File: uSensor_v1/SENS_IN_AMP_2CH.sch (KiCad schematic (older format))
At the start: 19 parts, among them U16 TBD

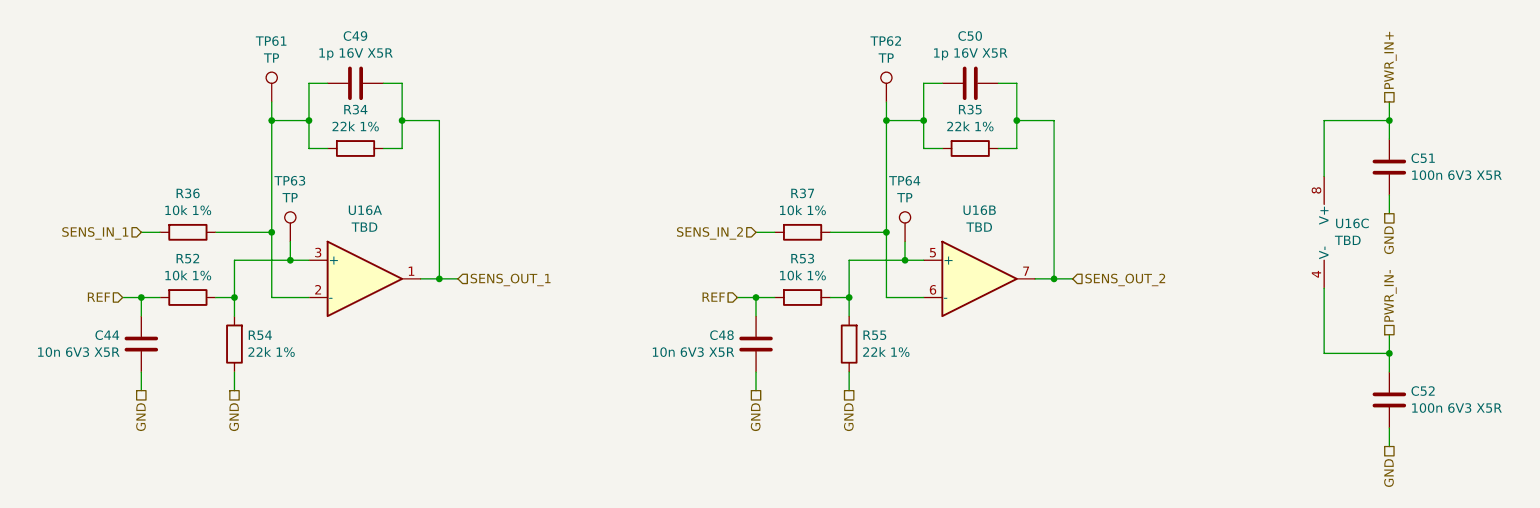
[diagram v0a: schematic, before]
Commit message: Layout in progress.
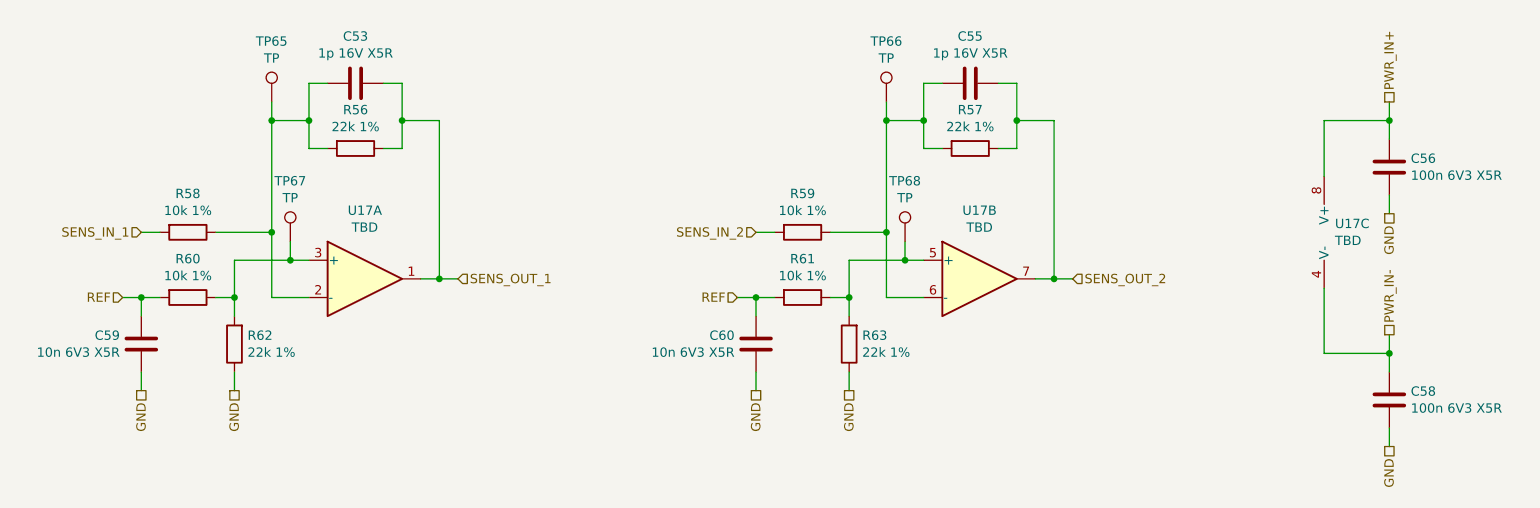
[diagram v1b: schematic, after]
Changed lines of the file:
@@
 AR Path="/5CFE311F/5C6F0205" Ref="R52"  Part="1"
 AR Path="/5E594B34/5C6F0205" Ref="R60"  Part="1"
-F 0 "R52" V 2443 3950 50  0000 C CNN
+F 0 "R60" V 2443 3950 50  0000 C CNN
 F 1 "10k 1%" V 2534 3950 50  0000 C CNN
 F 2 "Resistor_SMD:R_0603_1608Metric_Pad1.05x0.95mm_HandSolder" V 2580 3950 50  0001 C CNN
@@
 AR Path="/5CFE311F/5C6F020C" Ref="C49"  Part="1"
 AR Path="/5E594B34/5C6F020C" Ref="C53"  Part="1"
-F 0 "C49" V 3298 2800 50  0000 C CNN
+F 0 "C53" V 3298 2800 50  0000 C CNN
 F 1 "1p 16V X5R" V 3389 2800 50  0000 C CNN
 F 2 "Capacitor_SMD:C_0603_1608Metric_Pad1.05x0.95mm_HandSolder" H 3588 2650 50  0001 C CNN
@@
 AR Path="/5CFE311F/5C6F0213" Ref="R54"  Part="1"
 AR Path="/5E594B34/5C6F0213" Ref="R62"  Part="1"
-F 0 "R54" H 2830 4154 50  0000 R CNN
+F 0 "R62" H 2830 4154 50  0000 R CNN
 F 1 "22k 1%" H 2830 4245 50  0000 R CNN
 F 2 "Resistor_SMD:R_0603_1608Metric_Pad1.05x0.95mm_HandSolder" V 2830 4200 50  0001 C CNN
@@
 AR Path="/5CFE311F/5C6F0221" Ref="R36"  Part="1"
 AR Path="/5E594B34/5C6F0221" Ref="R58"  Part="1"
-F 0 "R36" V 2443 3600 50  0000 C CNN
+F 0 "R58" V 2443 3600 50  0000 C CNN
 F 1 "10k 1%" V 2534 3600 50  0000 C CNN
 F 2 "Resistor_SMD:R_0603_1608Metric_Pad1.05x0.95mm_HandSolder" V 2580 3600 50  0001 C CNN
@@
 AR Path="/5CFE311F/5C6F0228" Ref="R34"  Part="1"
 AR Path="/5E594B34/5C6F0228" Ref="R56"  Part="1"
-F 0 "R34" V 3343 3150 50  0000 C CNN
+F 0 "R56" V 3343 3150 50  0000 C CNN
 F 1 "22k 1%" V 3434 3150 50  0000 C CNN
 F 2 "Resistor_SMD:R_0603_1608Metric_Pad1.05x0.95mm_HandSolder" V 3480 3150 50  0001 C CNN
@@
 AR Path="/5CFE311F/5D2C6388" Ref="TP61"  Part="1"
 AR Path="/5E594B34/5D2C6388" Ref="TP65"  Part="1"
-F 0 "TP61" H 3100 3225 50  0000 C CNN
+F 0 "TP65" H 3100 3225 50  0000 C CNN
 F 1 "TP" H 3100 3134 50  0000 C CNN
 F 2 "Sentisa-Connectors:TestPoint_Probe_1.0mmDiameter_0.6mmDrill" H 3300 2900 50  0001 C CNN
@@
 AR Path="/5CFE311F/5D2C69C6" Ref="TP63"  Part="1"
 AR Path="/5E594B34/5D2C69C6" Ref="TP67"  Part="1"
-F 0 "TP63" H 3200 3975 50  0000 C CNN
+F 0 "TP67" H 3200 3975 50  0000 C CNN
 F 1 "TP" H 3200 3884 50  0000 C CNN
 F 2 "Sentisa-Connectors:TestPoint_Probe_1.0mmDiameter_0.6mmDrill" H 3400 3650 50  0001 C CNN
@@
 AR Path="/5CFE311F/5D1D3C08" Ref="R53"  Part="1"
 AR Path="/5E594B34/5D1D3C08" Ref="R61"  Part="1"
-F 0 "R53" V 5743 3950 50  0000 C CNN
+F 0 "R61" V 5743 3950 50  0000 C CNN
 F 1 "10k 1%" V 5834 3950 50  0000 C CNN
 F 2 "Resistor_SMD:R_0603_1608Metric_Pad1.05x0.95mm_HandSolder" V 5880 3950 50  0001 C CNN
@@
 AR Path="/5CFE311F/5D1D3C0F" Ref="C50"  Part="1"
 AR Path="/5E594B34/5D1D3C0F" Ref="C55"  Part="1"
-F 0 "C50" V 6598 2800 50  0000 C CNN
+F 0 "C55" V 6598 2800 50  0000 C CNN
 F 1 "1p 16V X5R" V 6689 2800 50  0000 C CNN
 F 2 "Capacitor_SMD:C_0603_1608Metric_Pad1.05x0.95mm_HandSolder" H 6888 2650 50  0001 C CNN
@@
 AR Path="/5CFE311F/5D1D3C16" Ref="R55"  Part="1"
 AR Path="/5E594B34/5D1D3C16" Ref="R63"  Part="1"
-F 0 "R55" H 6130 4154 50  0000 R CNN
+F 0 "R63" H 6130 4154 50  0000 R CNN
 F 1 "22k 1%" H 6130 4245 50  0000 R CNN
 F 2 "Resistor_SMD:R_0603_1608Metric_Pad1.05x0.95mm_HandSolder" V 6130 4200 50  0001 C CNN
@@
 AR Path="/5CFE311F/5D1D3C22" Ref="R37"  Part="1"
 AR Path="/5E594B34/5D1D3C22" Ref="R59"  Part="1"
-F 0 "R37" V 5743 3600 50  0000 C CNN
+F 0 "R59" V 5743 3600 50  0000 C CNN
 F 1 "10k 1%" V 5834 3600 50  0000 C CNN
 F 2 "Resistor_SMD:R_0603_1608Metric_Pad1.05x0.95mm_HandSolder" V 5880 3600 50  0001 C CNN
@@
 AR Path="/5CFE311F/5D1D3C29" Ref="R35"  Part="1"
 AR Path="/5E594B34/5D1D3C29" Ref="R57"  Part="1"
-F 0 "R35" V 6643 3150 50  0000 C CNN
+F 0 "R57" V 6643 3150 50  0000 C CNN
 F 1 "22k 1%" V 6734 3150 50  0000 C CNN
 F 2 "Resistor_SMD:R_0603_1608Metric_Pad1.05x0.95mm_HandSolder" V 6780 3150 50  0001 C CNN
@@
 AR Path="/5CFE311F/5D1D3C38" Ref="C51"  Part="1"
 AR Path="/5E594B34/5D1D3C38" Ref="C56"  Part="1"
-F 0 "C51" H 9215 3296 50  0000 L CNN
+F 0 "C56" H 9215 3296 50  0000 L CNN
 F 1 "100n 6V3 X5R" H 9215 3205 50  0000 L CNN
 F 2 "Capacitor_SMD:C_0603_1608Metric_Pad1.05x0.95mm_HandSolder" H 9138 3100 50  0001 C CNN
@@
 AR Path="/5CFE311F/5D1D3C3F" Ref="C52"  Part="1"
 AR Path="/5E594B34/5D1D3C3F" Ref="C58"  Part="1"
-F 0 "C52" H 9215 4546 50  0000 L CNN
+F 0 "C58" H 9215 4546 50  0000 L CNN
 F 1 "100n 6V3 X5R" H 9215 4455 50  0000 L CNN
 F 2 "Capacitor_SMD:C_0603_1608Metric_Pad1.05x0.95mm_HandSolder" H 9138 4350 50  0001 C CNN
@@
 AR Path="/5CFE311F/5D1D3C6C" Ref="TP62"  Part="1"
 AR Path="/5E594B34/5D1D3C6C" Ref="TP66"  Part="1"
-F 0 "TP62" H 6400 3225 50  0000 C CNN
+F 0 "TP66" H 6400 3225 50  0000 C CNN
 F 1 "TP" H 6400 3134 50  0000 C CNN
 F 2 "Sentisa-Connectors:TestPoint_Probe_1.0mmDiameter_0.6mmDrill" H 6600 2900 50  0001 C CNN
@@
 AR Path="/5CFE311F/5D1D3C73" Ref="TP64"  Part="1"
 AR Path="/5E594B34/5D1D3C73" Ref="TP68"  Part="1"
-F 0 "TP64" H 6500 3975 50  0000 C CNN
+F 0 "TP68" H 6500 3975 50  0000 C CNN
 F 1 "TP" H 6500 3884 50  0000 C CNN
 F 2 "Sentisa-Connectors:TestPoint_Probe_1.0mmDiameter_0.6mmDrill" H 6700 3650 50  0001 C CNN
@@
 AR Path="/5CFE311F/5F717FB4" Ref="U16"  Part="1"
 AR Path="/5E594B34/5F717FB4" Ref="U17"  Part="1"
-F 0 "U16" H 3600 4217 50  0000 C CNN
+F 0 "U17" H 3600 4217 50  0000 C CNN
 F 1 "TBD" H 3600 4126 50  0000 C CNN
 F 2 "Sentisa-IC:SO-8" H 3600 3850 50  0001 C CNN
@@
 AR Path="/5CFE311F/5F718017" Ref="U16"  Part="2"
 AR Path="/5E594B34/5F718017" Ref="U17"  Part="2"
-F 0 "U16" H 6900 4217 50  0000 C CNN
+F 0 "U17" H 6900 4217 50  0000 C CNN
 F 1 "TBD" H 6900 4126 50  0000 C CNN
 F 2 "Sentisa-IC:SO-8" H 6900 3850 50  0001 C CNN
@@
 AR Path="/5CFE311F/5F7180AE" Ref="U16"  Part="3"
 AR Path="/5E594B34/5F7180AE" Ref="U17"  Part="3"
-F 0 "U16" H 8808 3646 50  0000 L CNN
+F 0 "U17" H 8808 3646 50  0000 L CNN
 F 1 "TBD" H 8808 3555 50  0000 L CNN
 F 2 "Sentisa-IC:SO-8" H 8850 3600 50  0001 C CNN
@@
 AR Path="/5E594B34/5D0CECC5" Ref="C60"  Part="1"
 AR Path="/5CFE311F/5D0CECC5" Ref="C48"  Part="1"
-F 0 "C48" H 5585 4246 50  0000 R CNN
+F 0 "C60" H 5585 4246 50  0000 R CNN
 F 1 "10n 6V3 X5R" H 5585 4155 50  0000 R CNN
 F 2 "Capacitor_SMD:C_0603_1608Metric_Pad1.05x0.95mm_HandSolder" H 5738 4050 50  0001 C CNN
@@
 AR Path="/5E594B34/5D0D3A39" Ref="C59"  Part="1"
 AR Path="/5CFE311F/5D0D3A39" Ref="C44"  Part="1"
-F 0 "C44" H 2285 4246 50  0000 R CNN
+F 0 "C59" H 2285 4246 50  0000 R CNN
 F 1 "10n 6V3 X5R" H 2285 4155 50  0000 R CNN
 F 2 "Capacitor_SMD:C_0603_1608Metric_Pad1.05x0.95mm_HandSolder" H 2438 4050 50  0001 C CNN

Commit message: Connection done.
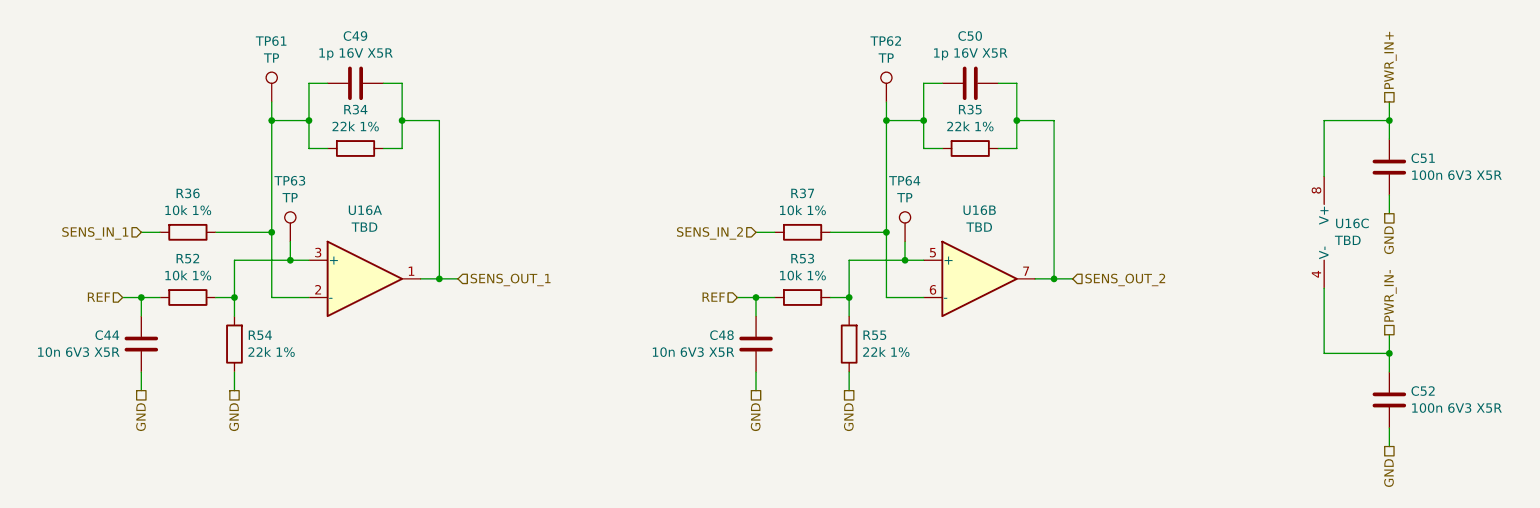
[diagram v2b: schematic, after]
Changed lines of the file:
@@
 AR Path="/5CFE311F/5C6F0205" Ref="R52"  Part="1"
 AR Path="/5E594B34/5C6F0205" Ref="R60"  Part="1"
-F 0 "R60" V 2443 3950 50  0000 C CNN
+F 0 "R52" V 2443 3950 50  0000 C CNN
 F 1 "10k 1%" V 2534 3950 50  0000 C CNN
 F 2 "Resistor_SMD:R_0603_1608Metric_Pad1.05x0.95mm_HandSolder" V 2580 3950 50  0001 C CNN
@@
 AR Path="/5CFE311F/5C6F020C" Ref="C49"  Part="1"
 AR Path="/5E594B34/5C6F020C" Ref="C53"  Part="1"
-F 0 "C53" V 3298 2800 50  0000 C CNN
+F 0 "C49" V 3298 2800 50  0000 C CNN
 F 1 "1p 16V X5R" V 3389 2800 50  0000 C CNN
 F 2 "Capacitor_SMD:C_0603_1608Metric_Pad1.05x0.95mm_HandSolder" H 3588 2650 50  0001 C CNN
@@
 AR Path="/5CFE311F/5C6F0213" Ref="R54"  Part="1"
 AR Path="/5E594B34/5C6F0213" Ref="R62"  Part="1"
-F 0 "R62" H 2830 4154 50  0000 R CNN
+F 0 "R54" H 2830 4154 50  0000 R CNN
 F 1 "22k 1%" H 2830 4245 50  0000 R CNN
 F 2 "Resistor_SMD:R_0603_1608Metric_Pad1.05x0.95mm_HandSolder" V 2830 4200 50  0001 C CNN
@@
 AR Path="/5CFE311F/5C6F0221" Ref="R36"  Part="1"
 AR Path="/5E594B34/5C6F0221" Ref="R58"  Part="1"
-F 0 "R58" V 2443 3600 50  0000 C CNN
+F 0 "R36" V 2443 3600 50  0000 C CNN
 F 1 "10k 1%" V 2534 3600 50  0000 C CNN
 F 2 "Resistor_SMD:R_0603_1608Metric_Pad1.05x0.95mm_HandSolder" V 2580 3600 50  0001 C CNN
@@
 AR Path="/5CFE311F/5C6F0228" Ref="R34"  Part="1"
 AR Path="/5E594B34/5C6F0228" Ref="R56"  Part="1"
-F 0 "R56" V 3343 3150 50  0000 C CNN
+F 0 "R34" V 3343 3150 50  0000 C CNN
 F 1 "22k 1%" V 3434 3150 50  0000 C CNN
 F 2 "Resistor_SMD:R_0603_1608Metric_Pad1.05x0.95mm_HandSolder" V 3480 3150 50  0001 C CNN
@@
 AR Path="/5CFE311F/5D2C6388" Ref="TP61"  Part="1"
 AR Path="/5E594B34/5D2C6388" Ref="TP65"  Part="1"
-F 0 "TP65" H 3100 3225 50  0000 C CNN
+F 0 "TP61" H 3100 3225 50  0000 C CNN
 F 1 "TP" H 3100 3134 50  0000 C CNN
 F 2 "Sentisa-Connectors:TestPoint_Probe_1.0mmDiameter_0.6mmDrill" H 3300 2900 50  0001 C CNN
@@
 AR Path="/5CFE311F/5D2C69C6" Ref="TP63"  Part="1"
 AR Path="/5E594B34/5D2C69C6" Ref="TP67"  Part="1"
-F 0 "TP67" H 3200 3975 50  0000 C CNN
+F 0 "TP63" H 3200 3975 50  0000 C CNN
 F 1 "TP" H 3200 3884 50  0000 C CNN
 F 2 "Sentisa-Connectors:TestPoint_Probe_1.0mmDiameter_0.6mmDrill" H 3400 3650 50  0001 C CNN
@@
 AR Path="/5CFE311F/5D1D3C08" Ref="R53"  Part="1"
 AR Path="/5E594B34/5D1D3C08" Ref="R61"  Part="1"
-F 0 "R61" V 5743 3950 50  0000 C CNN
+F 0 "R53" V 5743 3950 50  0000 C CNN
 F 1 "10k 1%" V 5834 3950 50  0000 C CNN
 F 2 "Resistor_SMD:R_0603_1608Metric_Pad1.05x0.95mm_HandSolder" V 5880 3950 50  0001 C CNN
@@
 AR Path="/5CFE311F/5D1D3C0F" Ref="C50"  Part="1"
 AR Path="/5E594B34/5D1D3C0F" Ref="C55"  Part="1"
-F 0 "C55" V 6598 2800 50  0000 C CNN
+F 0 "C50" V 6598 2800 50  0000 C CNN
 F 1 "1p 16V X5R" V 6689 2800 50  0000 C CNN
 F 2 "Capacitor_SMD:C_0603_1608Metric_Pad1.05x0.95mm_HandSolder" H 6888 2650 50  0001 C CNN
@@
 AR Path="/5CFE311F/5D1D3C16" Ref="R55"  Part="1"
 AR Path="/5E594B34/5D1D3C16" Ref="R63"  Part="1"
-F 0 "R63" H 6130 4154 50  0000 R CNN
+F 0 "R55" H 6130 4154 50  0000 R CNN
 F 1 "22k 1%" H 6130 4245 50  0000 R CNN
 F 2 "Resistor_SMD:R_0603_1608Metric_Pad1.05x0.95mm_HandSolder" V 6130 4200 50  0001 C CNN
@@
 AR Path="/5CFE311F/5D1D3C22" Ref="R37"  Part="1"
 AR Path="/5E594B34/5D1D3C22" Ref="R59"  Part="1"
-F 0 "R59" V 5743 3600 50  0000 C CNN
+F 0 "R37" V 5743 3600 50  0000 C CNN
 F 1 "10k 1%" V 5834 3600 50  0000 C CNN
 F 2 "Resistor_SMD:R_0603_1608Metric_Pad1.05x0.95mm_HandSolder" V 5880 3600 50  0001 C CNN
@@
 AR Path="/5CFE311F/5D1D3C29" Ref="R35"  Part="1"
 AR Path="/5E594B34/5D1D3C29" Ref="R57"  Part="1"
-F 0 "R57" V 6643 3150 50  0000 C CNN
+F 0 "R35" V 6643 3150 50  0000 C CNN
 F 1 "22k 1%" V 6734 3150 50  0000 C CNN
 F 2 "Resistor_SMD:R_0603_1608Metric_Pad1.05x0.95mm_HandSolder" V 6780 3150 50  0001 C CNN
@@
 AR Path="/5CFE311F/5D1D3C38" Ref="C51"  Part="1"
 AR Path="/5E594B34/5D1D3C38" Ref="C56"  Part="1"
-F 0 "C56" H 9215 3296 50  0000 L CNN
+F 0 "C51" H 9215 3296 50  0000 L CNN
 F 1 "100n 6V3 X5R" H 9215 3205 50  0000 L CNN
 F 2 "Capacitor_SMD:C_0603_1608Metric_Pad1.05x0.95mm_HandSolder" H 9138 3100 50  0001 C CNN
@@
 AR Path="/5CFE311F/5D1D3C3F" Ref="C52"  Part="1"
 AR Path="/5E594B34/5D1D3C3F" Ref="C58"  Part="1"
-F 0 "C58" H 9215 4546 50  0000 L CNN
+F 0 "C52" H 9215 4546 50  0000 L CNN
 F 1 "100n 6V3 X5R" H 9215 4455 50  0000 L CNN
 F 2 "Capacitor_SMD:C_0603_1608Metric_Pad1.05x0.95mm_HandSolder" H 9138 4350 50  0001 C CNN
@@
 AR Path="/5CFE311F/5D1D3C6C" Ref="TP62"  Part="1"
 AR Path="/5E594B34/5D1D3C6C" Ref="TP66"  Part="1"
-F 0 "TP66" H 6400 3225 50  0000 C CNN
+F 0 "TP62" H 6400 3225 50  0000 C CNN
 F 1 "TP" H 6400 3134 50  0000 C CNN
 F 2 "Sentisa-Connectors:TestPoint_Probe_1.0mmDiameter_0.6mmDrill" H 6600 2900 50  0001 C CNN
@@
 AR Path="/5CFE311F/5D1D3C73" Ref="TP64"  Part="1"
 AR Path="/5E594B34/5D1D3C73" Ref="TP68"  Part="1"
-F 0 "TP68" H 6500 3975 50  0000 C CNN
+F 0 "TP64" H 6500 3975 50  0000 C CNN
 F 1 "TP" H 6500 3884 50  0000 C CNN
 F 2 "Sentisa-Connectors:TestPoint_Probe_1.0mmDiameter_0.6mmDrill" H 6700 3650 50  0001 C CNN
@@
 AR Path="/5CFE311F/5F717FB4" Ref="U16"  Part="1"
 AR Path="/5E594B34/5F717FB4" Ref="U17"  Part="1"
-F 0 "U17" H 3600 4217 50  0000 C CNN
+F 0 "U16" H 3600 4217 50  0000 C CNN
 F 1 "TBD" H 3600 4126 50  0000 C CNN
 F 2 "Sentisa-IC:SO-8" H 3600 3850 50  0001 C CNN
@@
 AR Path="/5CFE311F/5F718017" Ref="U16"  Part="2"
 AR Path="/5E594B34/5F718017" Ref="U17"  Part="2"
-F 0 "U17" H 6900 4217 50  0000 C CNN
+F 0 "U16" H 6900 4217 50  0000 C CNN
 F 1 "TBD" H 6900 4126 50  0000 C CNN
 F 2 "Sentisa-IC:SO-8" H 6900 3850 50  0001 C CNN
@@
 AR Path="/5CFE311F/5F7180AE" Ref="U16"  Part="3"
 AR Path="/5E594B34/5F7180AE" Ref="U17"  Part="3"
-F 0 "U17" H 8808 3646 50  0000 L CNN
+F 0 "U16" H 8808 3646 50  0000 L CNN
 F 1 "TBD" H 8808 3555 50  0000 L CNN
 F 2 "Sentisa-IC:SO-8" H 8850 3600 50  0001 C CNN
@@
 AR Path="/5E594B34/5D0CECC5" Ref="C60"  Part="1"
 AR Path="/5CFE311F/5D0CECC5" Ref="C48"  Part="1"
-F 0 "C60" H 5585 4246 50  0000 R CNN
+F 0 "C48" H 5585 4246 50  0000 R CNN
 F 1 "10n 6V3 X5R" H 5585 4155 50  0000 R CNN
 F 2 "Capacitor_SMD:C_0603_1608Metric_Pad1.05x0.95mm_HandSolder" H 5738 4050 50  0001 C CNN
@@
 AR Path="/5E594B34/5D0D3A39" Ref="C59"  Part="1"
 AR Path="/5CFE311F/5D0D3A39" Ref="C44"  Part="1"
-F 0 "C59" H 2285 4246 50  0000 R CNN
+F 0 "C44" H 2285 4246 50  0000 R CNN
 F 1 "10n 6V3 X5R" H 2285 4155 50  0000 R CNN
 F 2 "Capacitor_SMD:C_0603_1608Metric_Pad1.05x0.95mm_HandSolder" H 2438 4050 50  0001 C CNN
